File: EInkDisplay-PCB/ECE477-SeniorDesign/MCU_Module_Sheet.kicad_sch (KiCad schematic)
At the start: 42 parts, among them J7 Conn_01x05, J8 Conn_01x05, U3 STM32L496ZGTxP, U7 PTS526 SK15 SMTR2 LFS, Y1 Y1

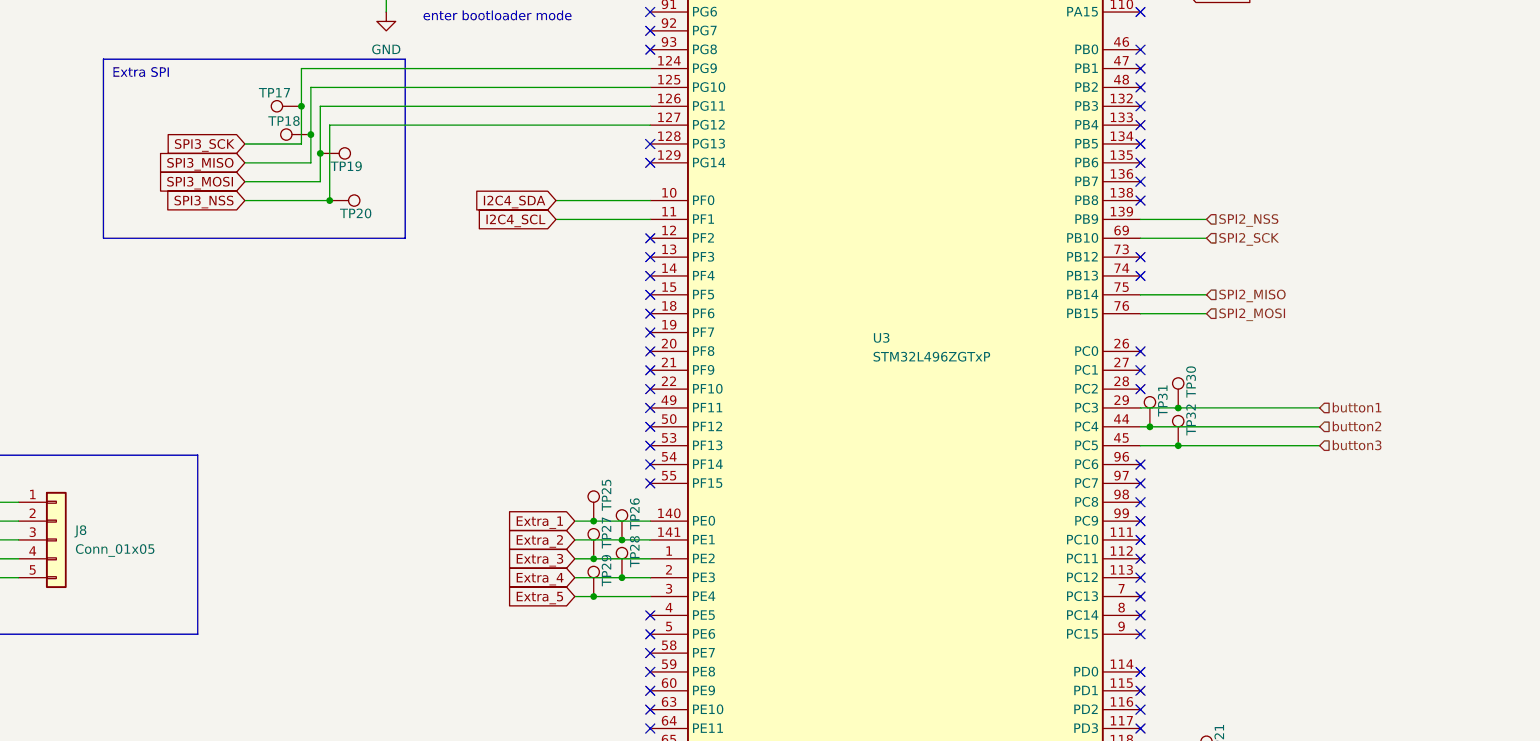
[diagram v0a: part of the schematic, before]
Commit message: whole lotta changes
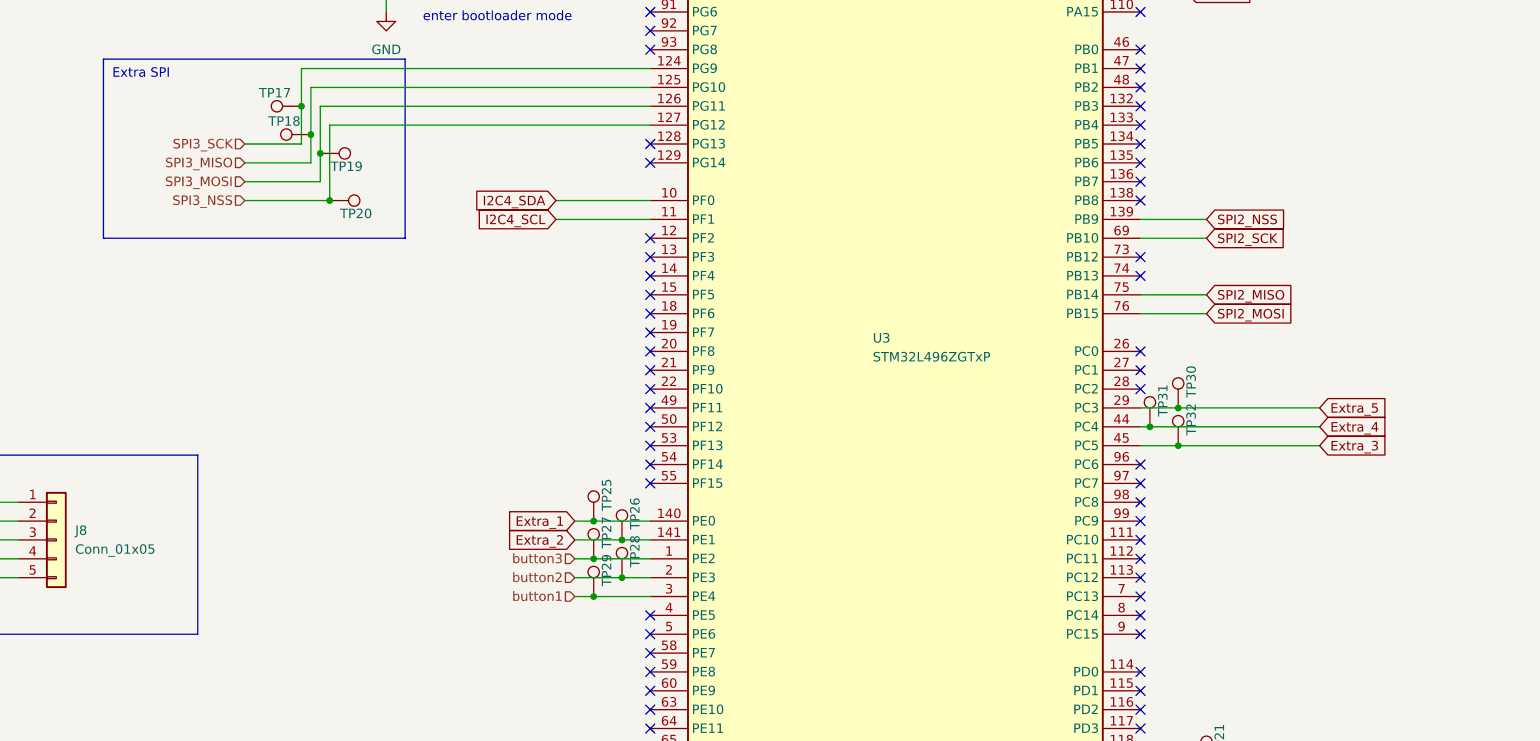
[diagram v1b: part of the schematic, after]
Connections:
- net Extra_3: now also TP32.1, U3.45 (PC5); no longer TP27.1, U3.1 (PE2)
- net Extra_4: now also TP31.1, U3.44 (PC4); no longer TP28.1, U3.2 (PE3)
- net Extra_5: now also TP30.1, U3.29 (PC3); no longer TP29.1, U3.3 (PE4)
- net button1: now also TP29.1, U3.3 (PE4); no longer TP30.1, U3.29 (PC3)
- net button2: now also TP28.1, U3.2 (PE3); no longer TP31.1, U3.44 (PC4)
- net button3: now also TP27.1, U3.1 (PE2); no longer TP32.1, U3.45 (PC5)

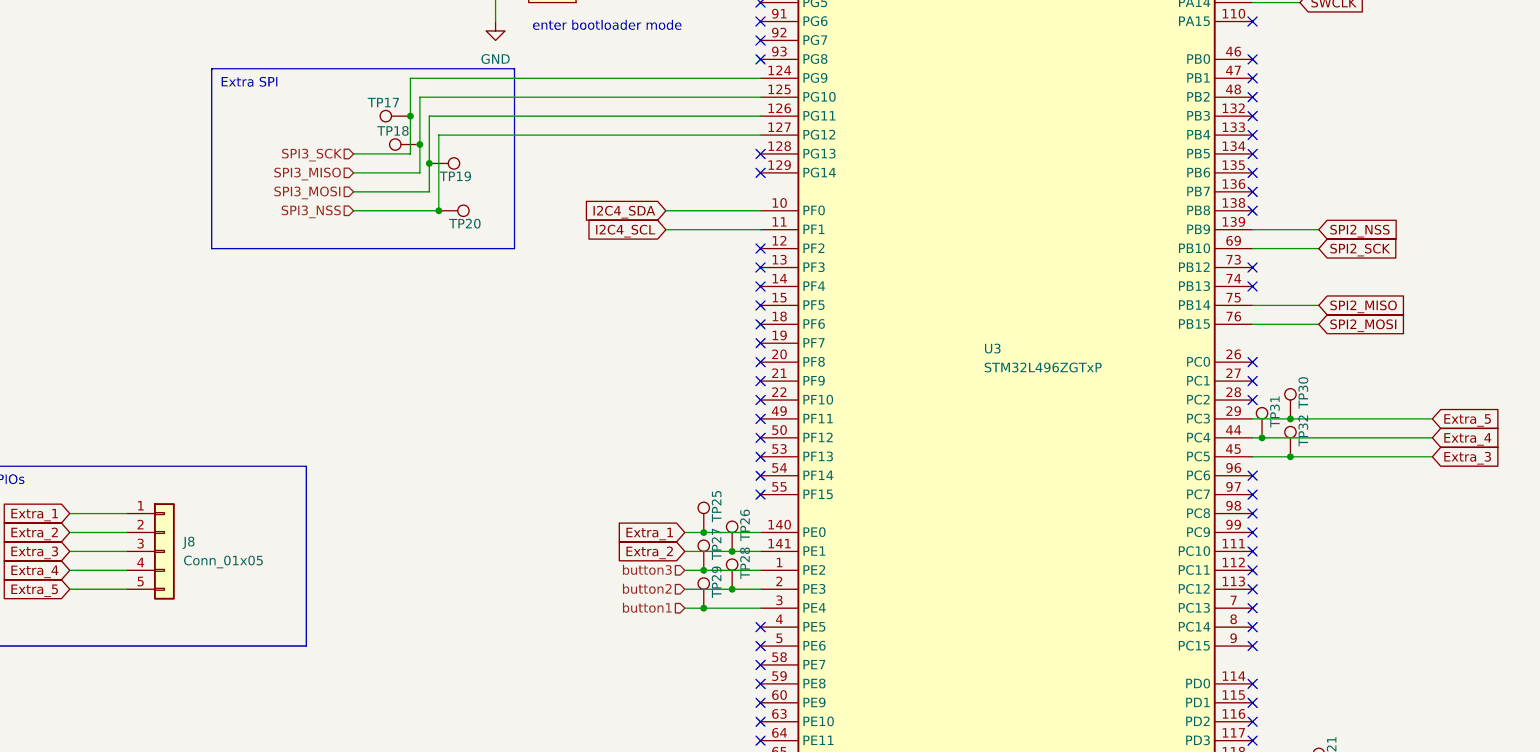
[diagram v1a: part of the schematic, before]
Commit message: pushing
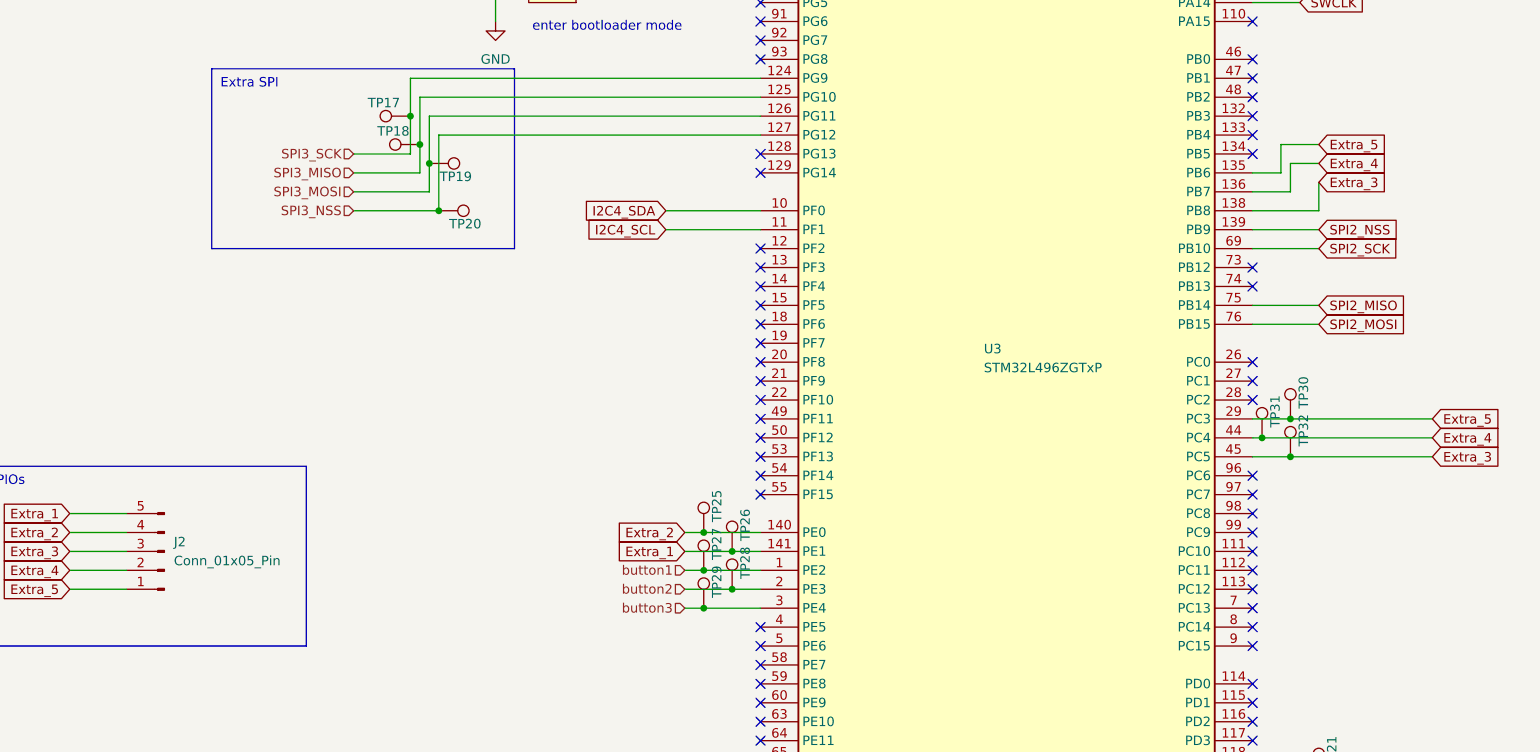
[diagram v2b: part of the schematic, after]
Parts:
- removed J8: Conn_01x05, symbol Connector_Generic:Conn_01x05
- added J2: Conn_01x05_Pin, Connector_PinHeader_1.00mm:PinHeader_1x05_P1.00mm_Vertical, symbol Connector:Conn_01x05_Pin
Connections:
- net Extra_1: now also TP26.1, U3.141 (PE1), J2.5 (Pin_5); no longer TP25.1, U3.140 (PE0)
- net Extra_2: now also TP25.1, U3.140 (PE0), J2.4 (Pin_4); no longer TP26.1, U3.141 (PE1)
- net Extra_3: now also U3.138 (PB8), J2.3 (Pin_3)
- net Extra_4: now also U3.136 (PB7), J2.2 (Pin_2)
- net Extra_5: now also U3.135 (PB6), J2.1 (Pin_1)
- net button1: now also TP27.1, U3.1 (PE2); no longer TP29.1, U3.3 (PE4)
- net button3: now also TP29.1, U3.3 (PE4); no longer TP27.1, U3.1 (PE2)
- no-connect marks 81 -> 78
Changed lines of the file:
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@@
 	)
 	(junction
+		(at 241.3 212.09)
+		(diameter 0)
+		(color 0 0 0 0)
+	)
+	(junction
 		(at 179.07 31.75)
 		(diameter 0)
@@
 	)
 	(junction
-		(at 241.3 212.09)
-		(diameter 0)
-		(color 0 0 0 0)
-	)
-	(junction
 		(at 218.44 36.83)
 		(diameter 0)
@@
 	)
 	(no_connect
-		(at 232.41 113.03)
-	)
-	(no_connect
 		(at 232.41 173.99)
 	)
@@
 	)
 	(no_connect
-		(at 232.41 115.57)
-	)
-	(no_connect
 		(at 232.41 219.71)
 	)
@@
 	)
 	(no_connect
-		(at 232.41 118.11)
-	)
-	(no_connect
 		(at 166.37 128.27)
 	)
@@
 	(wire
 		(pts
+			(xy 237.49 115.57) (xy 237.49 111.76)
+		)
+		(stroke
+			(width 0)
+			(type default)
+		)
+	)
+	(wire
+		(pts
 			(xy 187.96 31.75) (xy 191.77 31.75)
 		)
@@
 	(wire
 		(pts
+			(xy 232.41 113.03) (xy 236.22 113.03)
+		)
+		(stroke
+			(width 0)
+			(type default)
+		)
+	)
+	(wire
+		(pts
 			(xy 179.07 31.75) (xy 184.15 31.75)
 		)
@@
 	(wire
 		(pts
+			(xy 232.41 118.11) (xy 241.3 118.11)
+		)
+		(stroke
+			(width 0)
+			(type default)
+		)
+	)
+	(wire
+		(pts
 			(xy 223.52 36.83) (xy 228.6 36.83)
 		)
@@
 	(wire
 		(pts
+			(xy 237.49 111.76) (xy 241.3 111.76)
+		)
+		(stroke
+			(width 0)
+			(type default)
+		)
+	)
+	(wire
+		(pts
 			(xy 133.35 88.9) (xy 130.81 88.9)
 		)
@@
 	(wire
 		(pts
+			(xy 236.22 113.03) (xy 236.22 109.22)
+		)
+		(stroke
+			(width 0)
+			(type default)
+		)
+	)
+	(wire
+		(pts
 			(xy 138.43 54.61) (xy 146.05 54.61)
 		)
@@
 	(wire
 		(pts
+			(xy 236.22 109.22) (xy 241.3 109.22)
+		)
+		(stroke
+			(width 0)
+			(type default)
+		)
+	)
+	(wire
+		(pts
 			(xy 133.35 64.77) (xy 133.35 67.31)
 		)
@@
 	(wire
 		(pts
+			(xy 232.41 212.09) (xy 241.3 212.09)
+		)
+		(stroke
+			(width 0)
+			(type default)
+		)
+	)
+	(wire
+		(pts
 			(xy 232.41 146.05) (xy 237.49 146.05)
 		)
@@
 	(wire
 		(pts
-			(xy 232.41 212.09) (xy 241.3 212.09)
+			(xy 241.3 118.11) (xy 241.3 114.3)
 		)
 		(stroke
@@
 	(wire
 		(pts
+			(xy 232.41 115.57) (xy 237.49 115.57)
+		)
+		(stroke
+			(width 0)
+			(type default)
+		)
+	)
+	(wire
+		(pts
 			(xy 238.76 31.75) (xy 243.84 31.75)
 		)
@@
 		)
 	)
+	(global_label "Extra_5"
+		(shape input)
+		(at 241.3 109.22 0)
+		(fields_autoplaced yes)
+		(effects
+			(font
+				(size 1.27 1.27)
+			)
+			(justify left)
+		)
+		(property "Intersheetrefs" "${INTERSHEET_REFS}"
+			(at 251.3003 109.22 0)
+			(effects
+				(font
+					(size 1.27 1.27)
+				)
+				(justify left)
+				(hide yes)
+			)
+		)
+	)
 	(global_label "USART2_RX"
 		(shape input)
@@
 		)
 	)
-	(global_label "Extra_2"
+	(global_label "Extra_1"
 		(shape input)
 		(at 156.21 163.83 180)
@@
 		)
 	)
-	(global_label "Extra_1"
+	(global_label "Extra_2"
 		(shape input)
 		(at 156.21 161.29 180)
@@
 	(global_label "Extra_3"
 		(shape input)
+		(at 241.3 114.3 0)
+		(fields_autoplaced yes)
+		(effects
+			(font
+				(size 1.27 1.27)
+			)
+			(justify left)
+		)
+		(property "Intersheetrefs" "${INTERSHEET_REFS}"
+			(at 251.3003 114.3 0)
+			(effects
+				(font
+					(size 1.27 1.27)
+				)
+				(justify left)
+				(hide yes)
+			)
+		)
+	)
+	(global_label "Extra_3"
+		(shape input)
 		(at 256.54 151.13 0)
 		(fields_autoplaced yes)
@@
 		)
 	)
+	(global_label "Extra_4"
+		(shape input)
+		(at 241.3 111.76 0)
+		(fields_autoplaced yes)
+		(effects
+			(font
+				(size 1.27 1.27)
+			)
+			(justify left)
+		)
+		(property "Intersheetrefs" "${INTERSHEET_REFS}"
+			(at 251.3003 111.76 0)
+			(effects
+				(font
+					(size 1.27 1.27)
+				)
+				(justify left)
+				(hide yes)
+			)
+		)
+	)
 	(global_label "Extra_2"
 		(shape input)
@@
 		)
 	)
-	(hierarchical_label "button1"
+	(hierarchical_label "button3"
 		(shape input)
 		(at 156.21 171.45 180)
@@
 		)
 	)
-	(hierarchical_label "I2C2_SCL"
-		(shape input)
-		(at 281.94 212.09 0)
-		(effects
-			(font
-				(size 1.27 1.27)
-			)
-			(justify left)
-		)
-	)
 	(hierarchical_label "USART1_RX"
 		(shape input)
@@
 		)
 	)
-	(hierarchical_label "button3"
+	(hierarchical_label "button1"
 		(shape input)
 		(at 156.21 166.37 180)
@@
 		)
 	)
+	(hierarchical_label "I2C2_SCL"
+		(shape input)
+		(at 281.94 212.09 0)
+		(effects
+			(font
+				(size 1.27 1.27)
+			)
+			(justify left)
+		)
+	)
 	(hierarchical_label "USART1_TX"
 		(shape input)
@@
 	)
 	(symbol
-		(lib_id "Connector_Generic:Conn_01x05")
-		(at 86.36 163.83 0)
-		(unit 1)
-		(exclude_from_sim no)
-		(in_bom yes)
-		(on_board yes)
-		(dnp no)
-		(fields_autoplaced yes)
-		(property "Reference" "J8"
-			(at 88.9 162.5599 0)
-			(effects
-				(font
-					(size 1.27 1.27)
-				)
-				(justify left)
-			)
-		)
-		(property "Value" "Conn_01x05"
-			(at 88.9 165.0999 0)
-			(effects
-				(font
-					(size 1.27 1.27)
-				)
-				(justify left)
-			)
-		)
-		(property "Footprint" ""
-			(at 86.36 163.83 0)
-			(effects
-				(font
-					(size 1.27 1.27)
-				)
-				(hide yes)
-			)
-		)
-		(property "Datasheet" "~"
-			(at 86.36 163.83 0)
-			(effects
-				(font
-					(size 1.27 1.27)
-				)
-				(hide yes)
-			)
-		)
-		(property "Description" "Generic connector, single row, 01x05, script generated (kicad-library-utils/schlib/autogen/connector/)"
-			(at 86.36 163.83 0)
-			(effects
-				(font
-					(size 1.27 1.27)
-				)
-				(hide yes)
-			)
-		)
-		(pin "2"
-		)
-		(pin "1"
-		)
-		(pin "3"
-		)
-		(pin "4"
-		)
-		(pin "5"
-		)
-		(instances
-			(project "ECE477-SeniorDesign"
-				(path "/527ae649-08be-4368-9cf9-441ebba18eca/a47b6934-98dd-4056-b1df-1ab751d1c2a0"
-					(reference "J8")
-					(unit 1)
-				)
-			)
-		)
-	)
-	(symbol
 		(lib_id "power:GND")
 		(at 134.62 24.13 180)
@@
 					(unit 1)
 				)
+			)
+		)
+	)
+	(symbol
+		(lib_id "Connector:Conn_01x05_Pin")
+		(at 86.36 163.83 180)
+		(unit 1)
+		(exclude_from_sim no)
+		(in_bom yes)
+		(on_board yes)
+		(dnp no)
+		(fields_autoplaced yes)
+		(property "Reference" "J2"
+			(at 87.63 162.5599 0)
+			(effects
+				(font
+					(size 1.27 1.27)
+				)
+				(justify right)
+			)
+		)
+		(property "Value" "Conn_01x05_Pin"
+			(at 87.63 165.0999 0)
+			(effects
+				(font
+					(size 1.27 1.27)
+				)
+				(justify right)
+			)
+		)
+		(property "Footprint" "Connector_PinHeader_1.00mm:PinHeader_1x05_P1.00mm_Vertical"
+			(at 86.36 163.83 0)
+			(effects
+				(font
+					(size 1.27 1.27)
+				)
+				(hide yes)
+			)
+		)
+		(property "Datasheet" "~"
+			(at 86.36 163.83 0)
+			(effects
+				(font
+					(size 1.27 1.27)
+				)
+				(hide yes)
+			)
+		)
+		(property "Description" "Generic connector, single row, 01x05, script generated"
+			(at 86.36 163.83 0)
+			(effects
+				(font
+					(size 1.27 1.27)
+				)
+				(hide yes)
+			)
+		)
+		(pin "4"
+		)
+		(pin "5"
+		)
+		(pin "3"
+		)
+		(pin "2"
+		)
+		(pin "1"
+		)
+		(instances
+			(project ""
+				(path "/527ae649-08be-4368-9cf9-441ebba18eca/a47b6934-98dd-4056-b1df-1ab751d1c2a0"
+					(reference "J2")
+					(unit 1)
+				)
